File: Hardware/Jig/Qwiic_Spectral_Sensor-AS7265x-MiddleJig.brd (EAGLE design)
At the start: 35.6 x 40.6 mm, 93 parts, among them J2 Serial Interface, J5 Flash Programming, J8 PTH, U1 AS72651, U3 4MB Flash, U5 AS72653, U6 AS72652

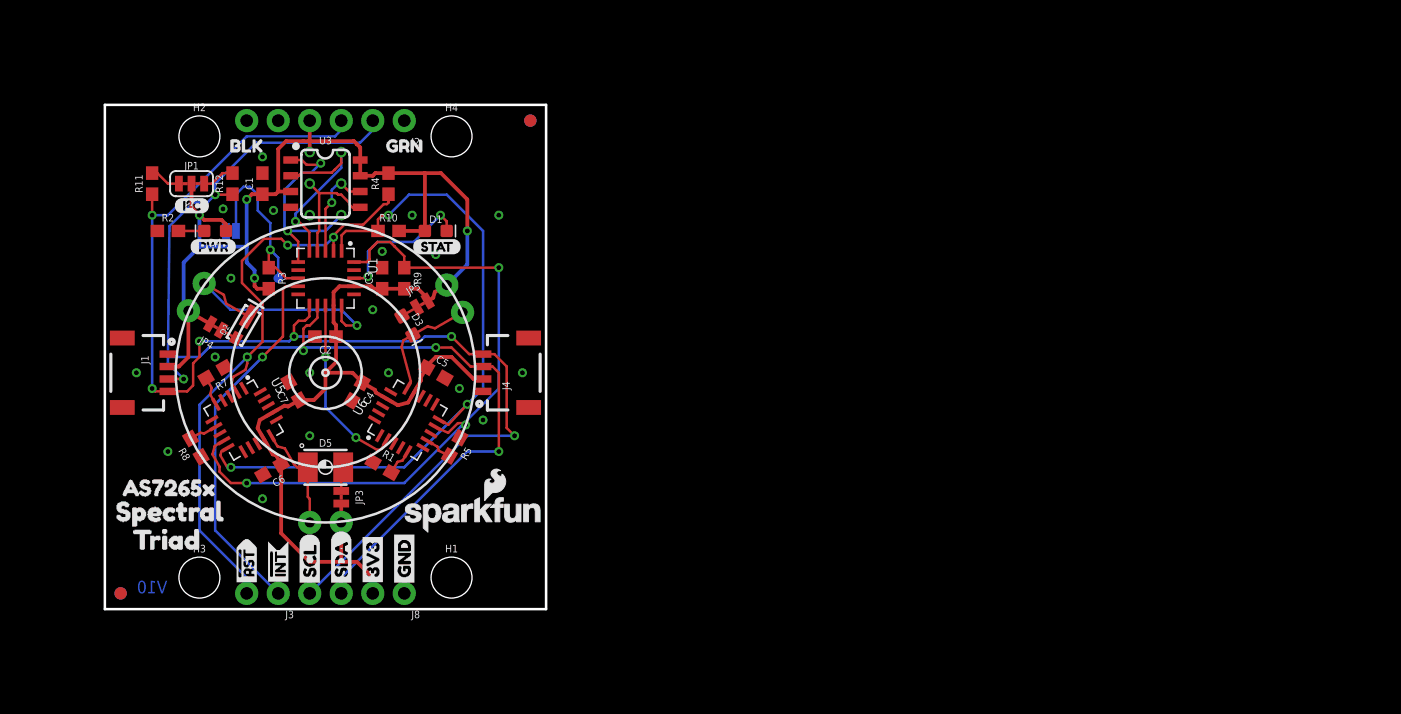
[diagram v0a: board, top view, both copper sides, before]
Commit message: Silk changes before panelization
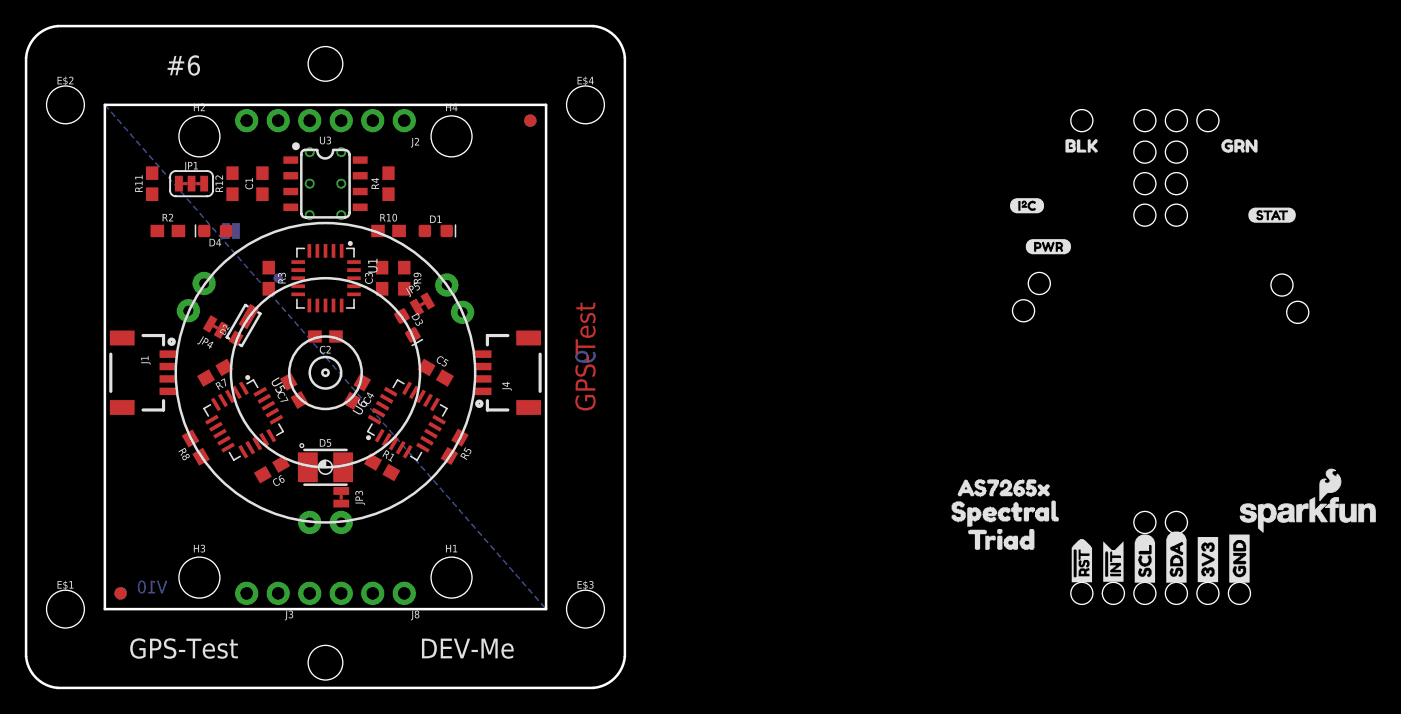
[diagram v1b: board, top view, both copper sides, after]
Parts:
- removed U$1, U$36, U$37: (no value), buzzard_labels (7):#0
- removed U$38, U$39, U$40: (no value), buzzard_labels (7):#1
- added E$1, E$2, E$3, E$4: (no value), SparkFun-Hardware:STAND-OFF-TIGHT
- added E$5, E$6: (no value), SparkFun-Hardware:NUBBIN_LOCKER
- D2: device SparkFun-LED:SUPER_BRIGHT_SMD_LED_3014 -> SparkX:SUPER_BRIGHT_SMD_LED_1206
- moved U$10 67.4 mm to (92.1, 31.8)
- moved FRAME1 67.3 mm to (55.9, -30.5)
- moved LOGO4 67.3 mm to (100.3, 2.54)
- moved U$11 67.3 mm to (68.2, 5.59)
- moved U$13 67.3 mm to (78.4, 7.87)
- moved U$17 67.3 mm to (78.7, 33.9)
- moved U$19 67.3 mm to (91.4, 34.8)
- moved U$2 67.3 mm to (72.9, 32.5)
- moved U$21 67.3 mm to (85.2, 34.4)
- moved U$22 67.3 mm to (88.6, 33.0)
- moved U$25 67.3 mm to (91.4, 1.65)
- moved U$26 67.3 mm to (86.4, 1.65)
- moved U$29 67.3 mm to (78.7, 1.52)
- moved U$30 67.3 mm to (91.4, 1.65)
- moved U$32 67.3 mm to (86.4, 1.65)
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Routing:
- net 3.3V: track 143.3 -> 0.00 mm, vias 4 -> 0
- net RX/SCL: track 99.0 -> 0.00 mm, vias 6 -> 0
- net TX/SDA: track 93.2 -> 0.00 mm, vias 5 -> 0
- net SDA_S: track 56.9 -> 0.00 mm, vias 3 -> 0
- net SCL_S: track 56.2 -> 0.00 mm, vias 3 -> 0
- net !RST: track 50.8 -> 0.00 mm, vias 3 -> 0
- net !INT: track 30.2 -> 0.00 mm, vias 1 -> 0
- net LED_DRV: track 21.0 -> 0.00 mm, vias 1 -> 0
- net !CS_EE: track 17.6 -> 0.00 mm, vias 2 -> 0
- net I2C_ENB: track 16.8 -> 0.00 mm, vias 1 -> 0
- net MISO: track 15.5 -> 0.00 mm, vias 1 -> 0
- net !RST-ADDR: track 14.9 -> 0.00 mm, vias 2 -> 0
- net N$2: track 11.8 -> 0.00 mm, vias 2 -> 0
- net MOSI: track 9.65 -> 0.00 mm
- net LED_DRV1: track 9.51 -> 0.00 mm
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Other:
- board size 35.6 x 40.6 mm -> 48.3 x 53.3 mm
- board text added: "#6"
- board text added: "6"
- board text added: "DEV-Me"
- board text added: "GPS-Test"
